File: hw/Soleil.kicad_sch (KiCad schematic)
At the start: 43 parts, among them J1 Conn_01x04, Q1 2N7002, SW1 SW_Push, U1 SPV1040TTR, U2 TPS61220DCK, U3 STM32G030F6Px, U4 ZJY200200-0154DAAMFGN

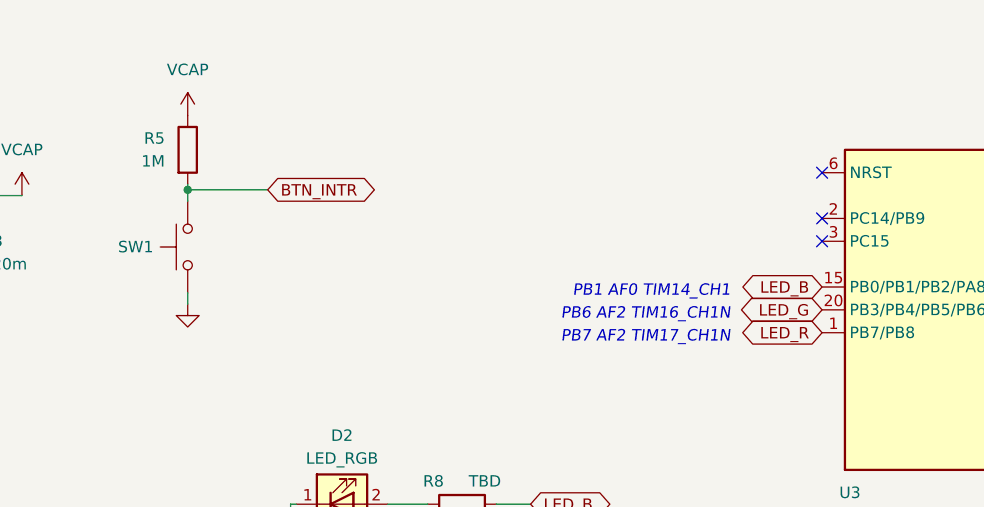
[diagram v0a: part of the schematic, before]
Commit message: Revise circuit board design; submit for fab
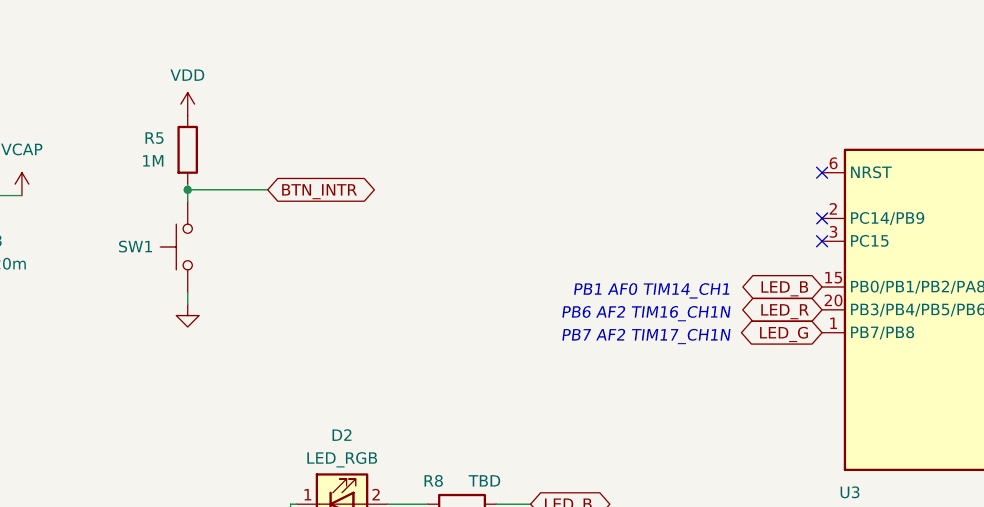
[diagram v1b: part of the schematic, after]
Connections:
- net LED_G: now also U3.1 (PB7/PB8); no longer U3.20 (PB3/PB4/PB5/PB6)
- net LED_R: now also U3.20 (PB3/PB4/PB5/PB6); no longer U3.1 (PB7/PB8)
- net VCAP: no longer R5.1
- net VDD: now also R5.1
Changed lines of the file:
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@@
     )
   )
-  (global_label "LED_R" (shape bidirectional) (at 190.5 54.61 180) (fields_autoplaced)
+  (global_label "LED_G" (shape bidirectional) (at 190.5 54.61 180) (fields_autoplaced)
     (effects (font (size 1.27 1.27)) (justify right))
     (property "Intersheetrefs" "${INTERSHEET_REFS}" (at 180.7188 54.61 0)
@@
     )
   )
-  (global_label "LED_G" (shape bidirectional) (at 190.5 52.07 180) (fields_autoplaced)
+  (global_label "LED_R" (shape bidirectional) (at 190.5 52.07 180) (fields_autoplaced)
     (effects (font (size 1.27 1.27)) (justify right))
     (property "Intersheetrefs" "${INTERSHEET_REFS}" (at 180.7188 52.07 0)
@@
         (path "/218ebbfa-f714-4191-a352-4c256789be77"
           (reference "C13") (unit 1)
+        )
+      )
+    )
+  )
+  (symbol (lib_id "power:VDD") (at 120.015 30.48 0) (unit 1)
+    (in_bom yes) (on_board yes) (dnp no) (fields_autoplaced)
+    (property "Reference" "#PWR011" (at 120.015 34.29 0)
+      (effects (font (size 1.27 1.27)) hide)
+    )
+    (property "Value" "VDD" (at 120.015 26.035 0)
+      (effects (font (size 1.27 1.27)))
+    )
+    (property "Footprint" "" (at 120.015 30.48 0)
+      (effects (font (size 1.27 1.27)) hide)
+    )
+    (property "Datasheet" "" (at 120.015 30.48 0)
+      (effects (font (size 1.27 1.27)) hide)
+    )
+    (pin "1")
+    (instances
+      (project "Soleil"
+        (path "/218ebbfa-f714-4191-a352-4c256789be77"
+          (reference "#PWR011") (unit 1)
         )
       )
@@
         )
       )
-    )
-  )
-  (symbol (lib_id "Soleil_symbols:VCAP") (at 120.015 30.48 0) (unit 1)
-    (in_bom yes) (on_board yes) (dnp no) (fields_autoplaced)
-    (property "Reference" "#PWR011" (at 120.015 34.29 0)
-      (effects (font (size 1.27 1.27)) hide)
-    )
-    (property "Value" "VCAP" (at 120.015 25.4 0)
-      (effects (font (size 1.27 1.27)))
-    )
-    (property "Footprint" "" (at 120.015 30.48 0)
-      (effects (font (size 1.27 1.27)) hide)
-    )
-    (property "Datasheet" "" (at 120.015 30.48 0)
-      (effects (font (size 1.27 1.27)) hide)
-    )
-    (pin "1")
-    (instances
-      (project "Soleil"
-        (path "/218ebbfa-f714-4191-a352-4c256789be77"
-          (reference "#PWR011") (unit 1)
-        )
-      )
